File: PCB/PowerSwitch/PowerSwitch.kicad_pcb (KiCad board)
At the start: 4 copper layers, 27 x 23.1 mm, 5 parts, among them J1 Conn_01x02_Pin, J2 Conn_01x02_Pin, J3 Conn_01x02_Socket, J4 Conn_01x02_Socket

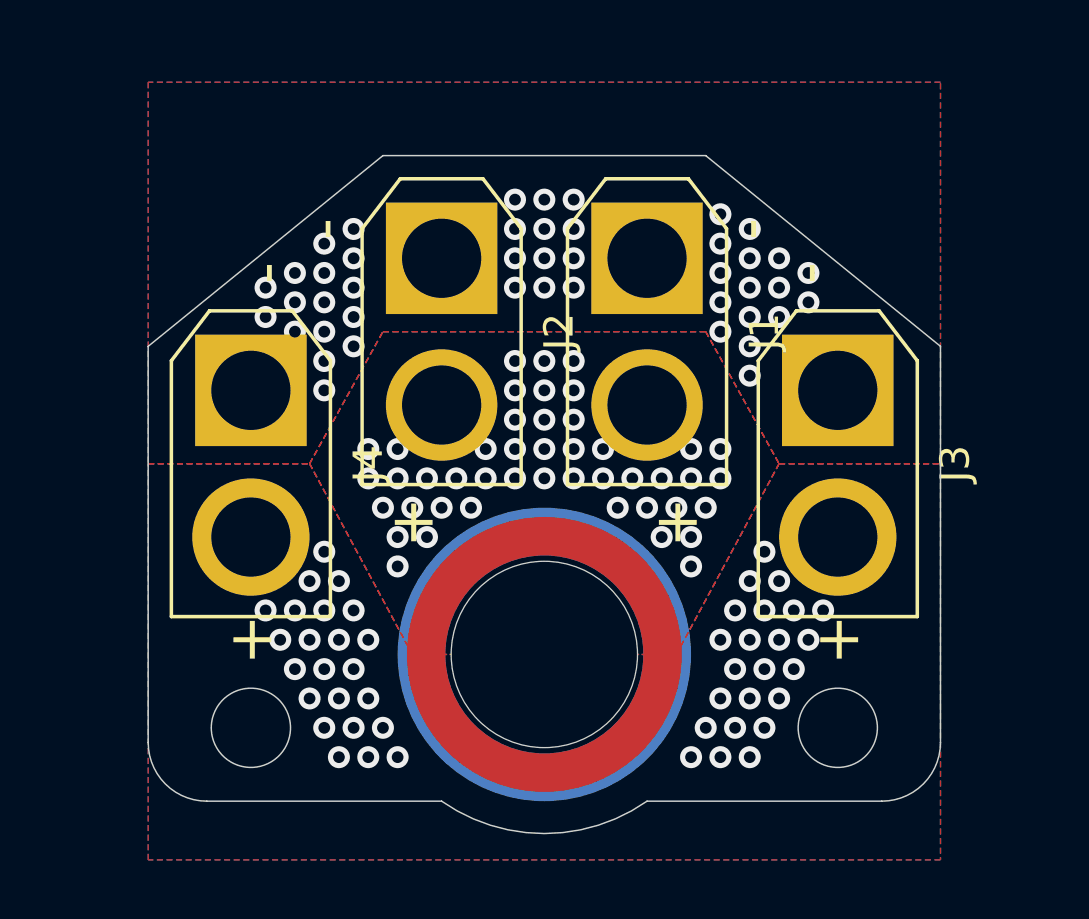
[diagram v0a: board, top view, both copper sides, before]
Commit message: angled xt30
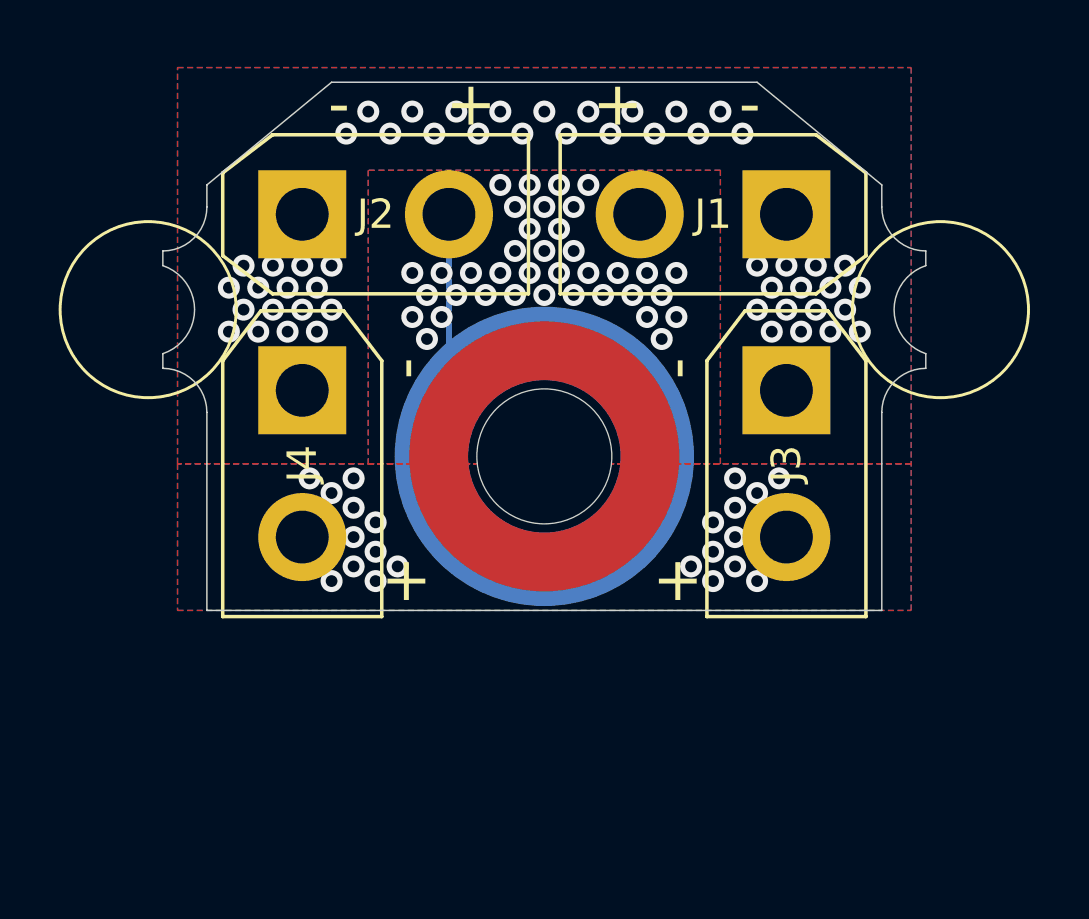
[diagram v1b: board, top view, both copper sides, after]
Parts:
- J1, J2: footprint Connector_AMASS:AMASS_XT30U-M_1x02_P5.0mm_Vertical -> Connector_AMASS:AMASS_XT30UPB-F_1x02_P5.0mm_Vertical
- J3, J4: footprint Connector_AMASS:AMASS_XT30U-F_1x02_P5.0mm_Vertical -> Connector_AMASS:AMASS_XT30UPB-F_1x02_P5.0mm_Vertical
- moved SW1 6.75 mm to (85.0, 73.2)
- moved J1 4.98 mm to (93.2, 65.0), turned to 180 degrees
- moved J2 4.98 mm to (76.8, 65.0), turned to 0 degrees
- moved J3 1.75 mm to (93.2, 71.0)
- moved J4 1.75 mm to (76.8, 71.0)
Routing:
- net /BATT: track 0.00 -> 9.43 mm, vias 45 -> 37
- net GND: vias 44 -> 51
- net /VCC: vias 46 -> 22
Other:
- board size 27 x 23.1 mm -> 26 x 18 mm
